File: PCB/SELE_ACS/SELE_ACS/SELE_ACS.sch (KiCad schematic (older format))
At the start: 20 parts, among them J1 AVR-ISP-6, J2 Input Cables, SW1 Button Reset, SW2 SW_DIP_x04, U1 ATmega328P-PU, U2 MAX485E, U3 LM7805_TO220, Y1 Crystal 8MHz

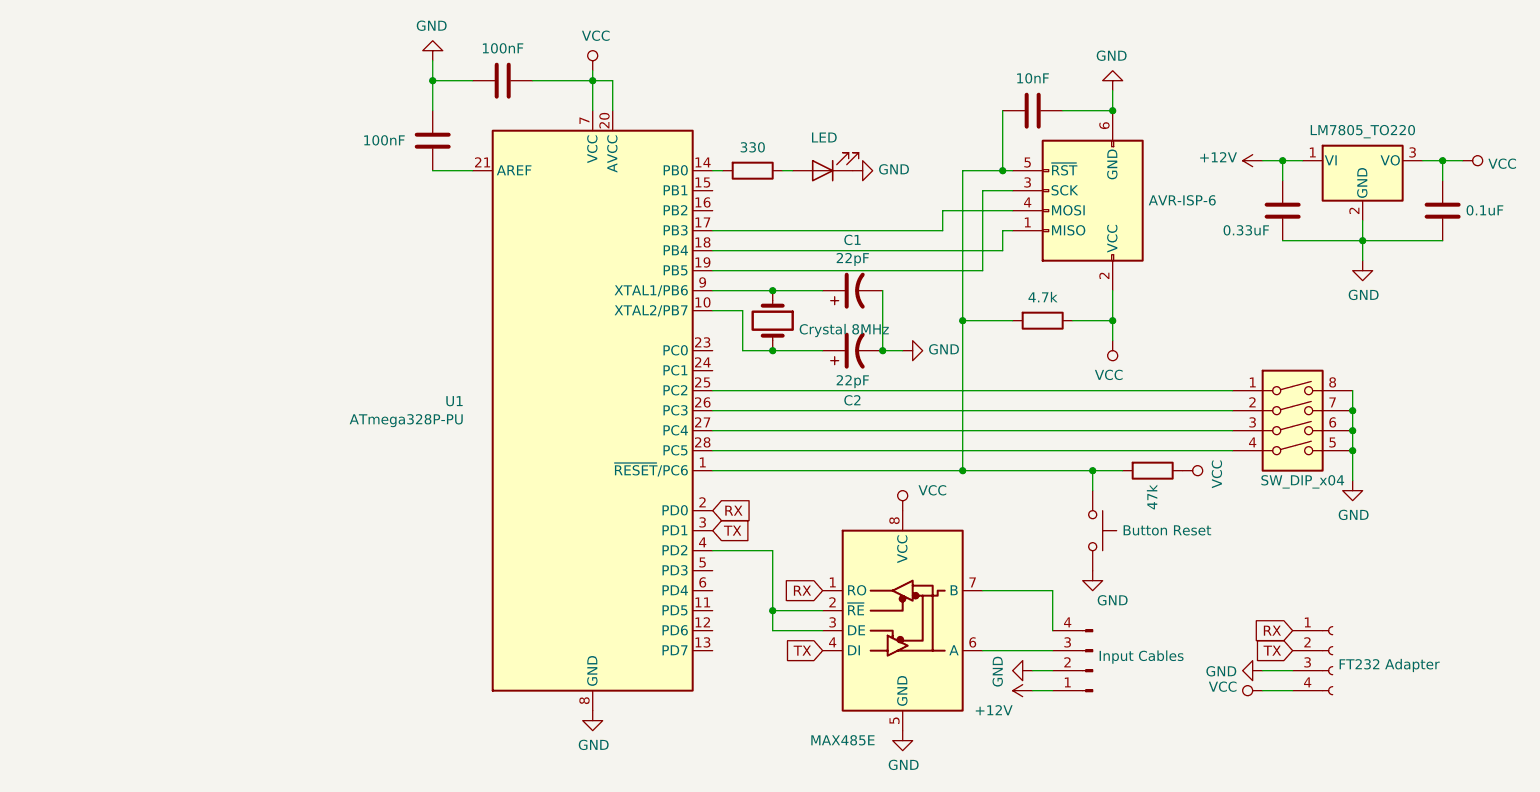
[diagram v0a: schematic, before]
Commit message: Add files via upload
pcbnew added
socket symbol, footprint and 3d model added
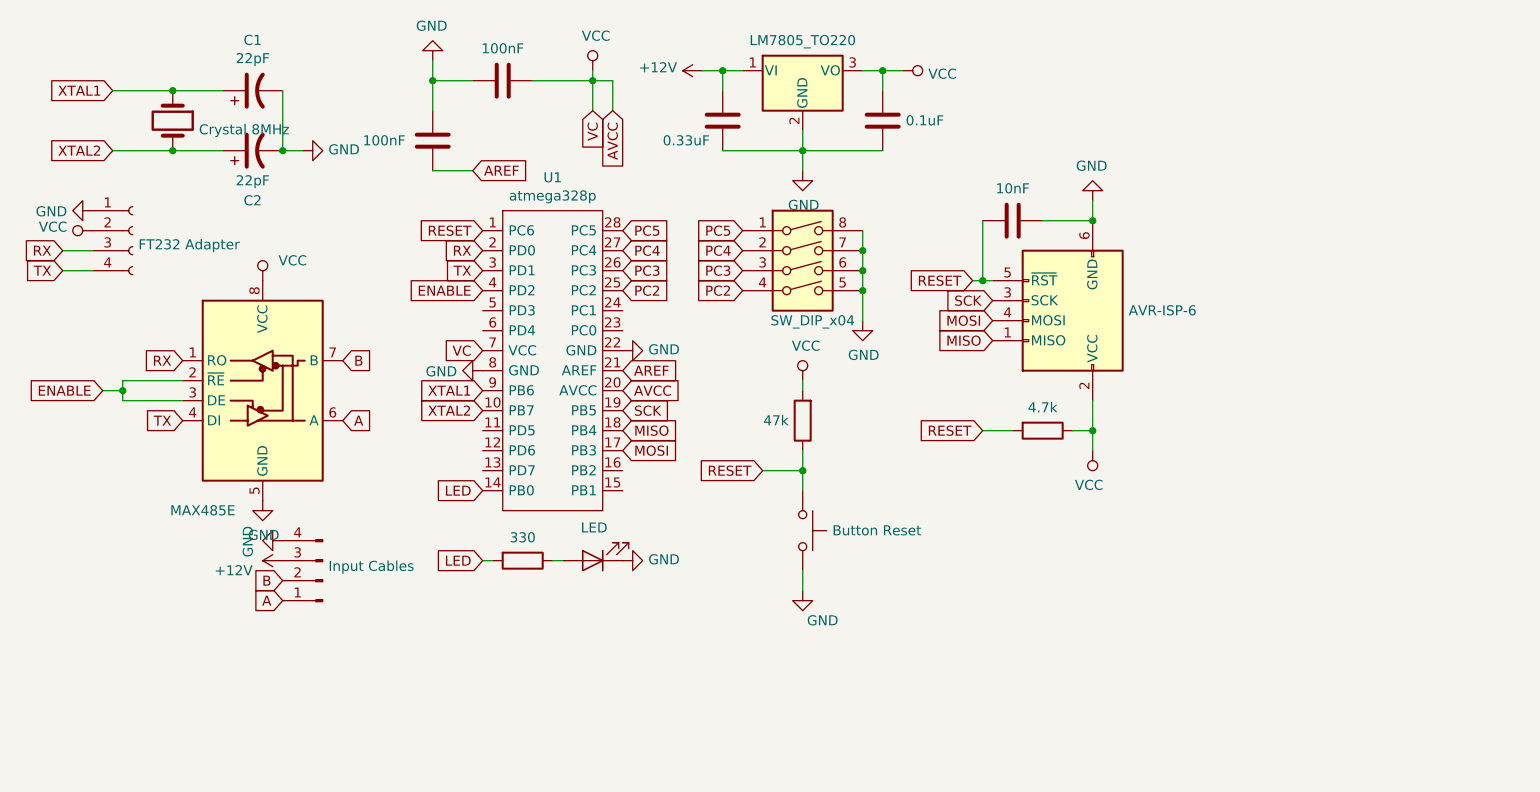
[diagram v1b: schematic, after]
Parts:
- removed U1: ATmega328P-PU, Package_DIP:DIP-28_W7.62mm, symbol MCU_Microchip_ATmega:ATmega328P-PU
- added U1: atmega328p, Package_DIP:DIP-28_W7.62mm, symbol SELE:atmega328p
- C1, C2: footprint (none) -> Capacitor_THT:CP_Radial_D4.0mm_P1.50mm
- C3, C4, C5, C6, C7: footprint (none) -> Capacitor_THT:C_Rect_L7.0mm_W2.0mm_P5.00mm
- D1: footprint (none) -> LED_THT:LED_D3.0mm
- J1: footprint (none) -> Connector_PinHeader_2.54mm:PinHeader_2x03_P2.54mm_Vertical
- J2: footprint (none) -> Connector_PinHeader_2.54mm:PinHeader_1x04_P2.54mm_Vertical
- J3: renamed from J?; footprint (none) -> Socket_Strips:Socket_Strip_Straight_1x04_Pitch2.54mm
- R1, R2, R3: footprint (none) -> Resistor_THT:R_Axial_DIN0207_L6.3mm_D2.5mm_P10.16mm_Horizontal
- SW1: footprint (none) -> Button_Switch_THT:SW_PUSH_6mm
- SW2: footprint (none) -> Button_Switch_THT:SW_DIP_SPSTx04_Slide_9.78x12.34mm_W7.62mm_P2.54mm
- U2: footprint (none) -> Package_DIP:DIP-8_W7.62mm
- Y1: footprint (none) -> Crystal:Crystal_HC49-U_Vertical
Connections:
- net +12V: now also J2.3 (Pin_3); no longer J2.1 (Pin_1)
- net GND: now also J2.4 (Pin_4), J3.1 (Pin_1), U1.22 (GND), U1.8 (GND); no longer J2.2 (Pin_2), J3.3 (Pin_3)
- net RX: now also J3.3 (Pin_3), U1.2 (PD0); no longer J3.1 (Pin_1)
- net TX: now also J3.4 (Pin_4), U1.3 (PD1); no longer J3.2 (Pin_2)
- net VCC: now also J3.2 (Pin_2), R3.2, U1.20 (AVCC), U1.7 (VCC); no longer J3.4 (Pin_4), R3.1
- net RESET: now reaches C5.2, J1.5 (~RST), R2.2, SW1.1
- net RESET: now also R3.1, U1.1 (PC6); no longer R3.2
- net XTAL2: now reaches C2.1, Y1.2
- net XTAL2: now also U1.10 (PB7)
- net LED: now reaches R1.2
- net LED: now also U1.14 (PB0)
- net MOSI: now reaches J1.4 (MOSI)
- net MOSI: now also U1.17 (PB3)
- net MISO: now reaches J1.1 (MISO)
- net MISO: now also U1.18 (PB4)
- net SCK: now reaches J1.3 (SCK)
- net SCK: now also U1.19 (PB5)
- net AREF: now reaches C3.1
- net AREF: now also U1.21 (AREF)
- net PC5: now reaches SW2.1
- net PC5: now also U1.28 (PC5)
- net PC4: now reaches SW2.2
- net PC4: now also U1.27 (PC4)
- net PC3: now reaches SW2.3
- net PC3: now also U1.26 (PC3)
- net PC2: now reaches SW2.4
- net PC2: now also U1.25 (PC2)
- net ENABLE: now reaches U2.2 (~RE), U2.3 (DE)
- net ENABLE: now also U1.4 (PD2)
- net XTAL1: now reaches C1.1, Y1.1
- net XTAL1: now also U1.9 (PB6)
- net A: now reaches U2.6 (A)
- net A: now also J2.1 (Pin_1); no longer J2.3 (Pin_3)
- net B: now reaches U2.7 (B)
- net B: now also J2.2 (Pin_2); no longer J2.4 (Pin_4)
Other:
- moved on the sheet: C1, C2
